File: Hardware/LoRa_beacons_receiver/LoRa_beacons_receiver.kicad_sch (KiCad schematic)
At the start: 44 parts, among them J1 Conn_Coaxial, J2 USB_C_Receptacle_USB2.0_16P, J3 I2C_Display, J4 ST-Link, J5 1PPS_out, J6 Conn_02x09_Counter_Clockwise, SW1 RST_button, SW2 BOOT_button, U1 Wio-E5, U2 CP2102N-Axx-xQFN28, U3 AP2112K-3.3, U5 74LVC1G17

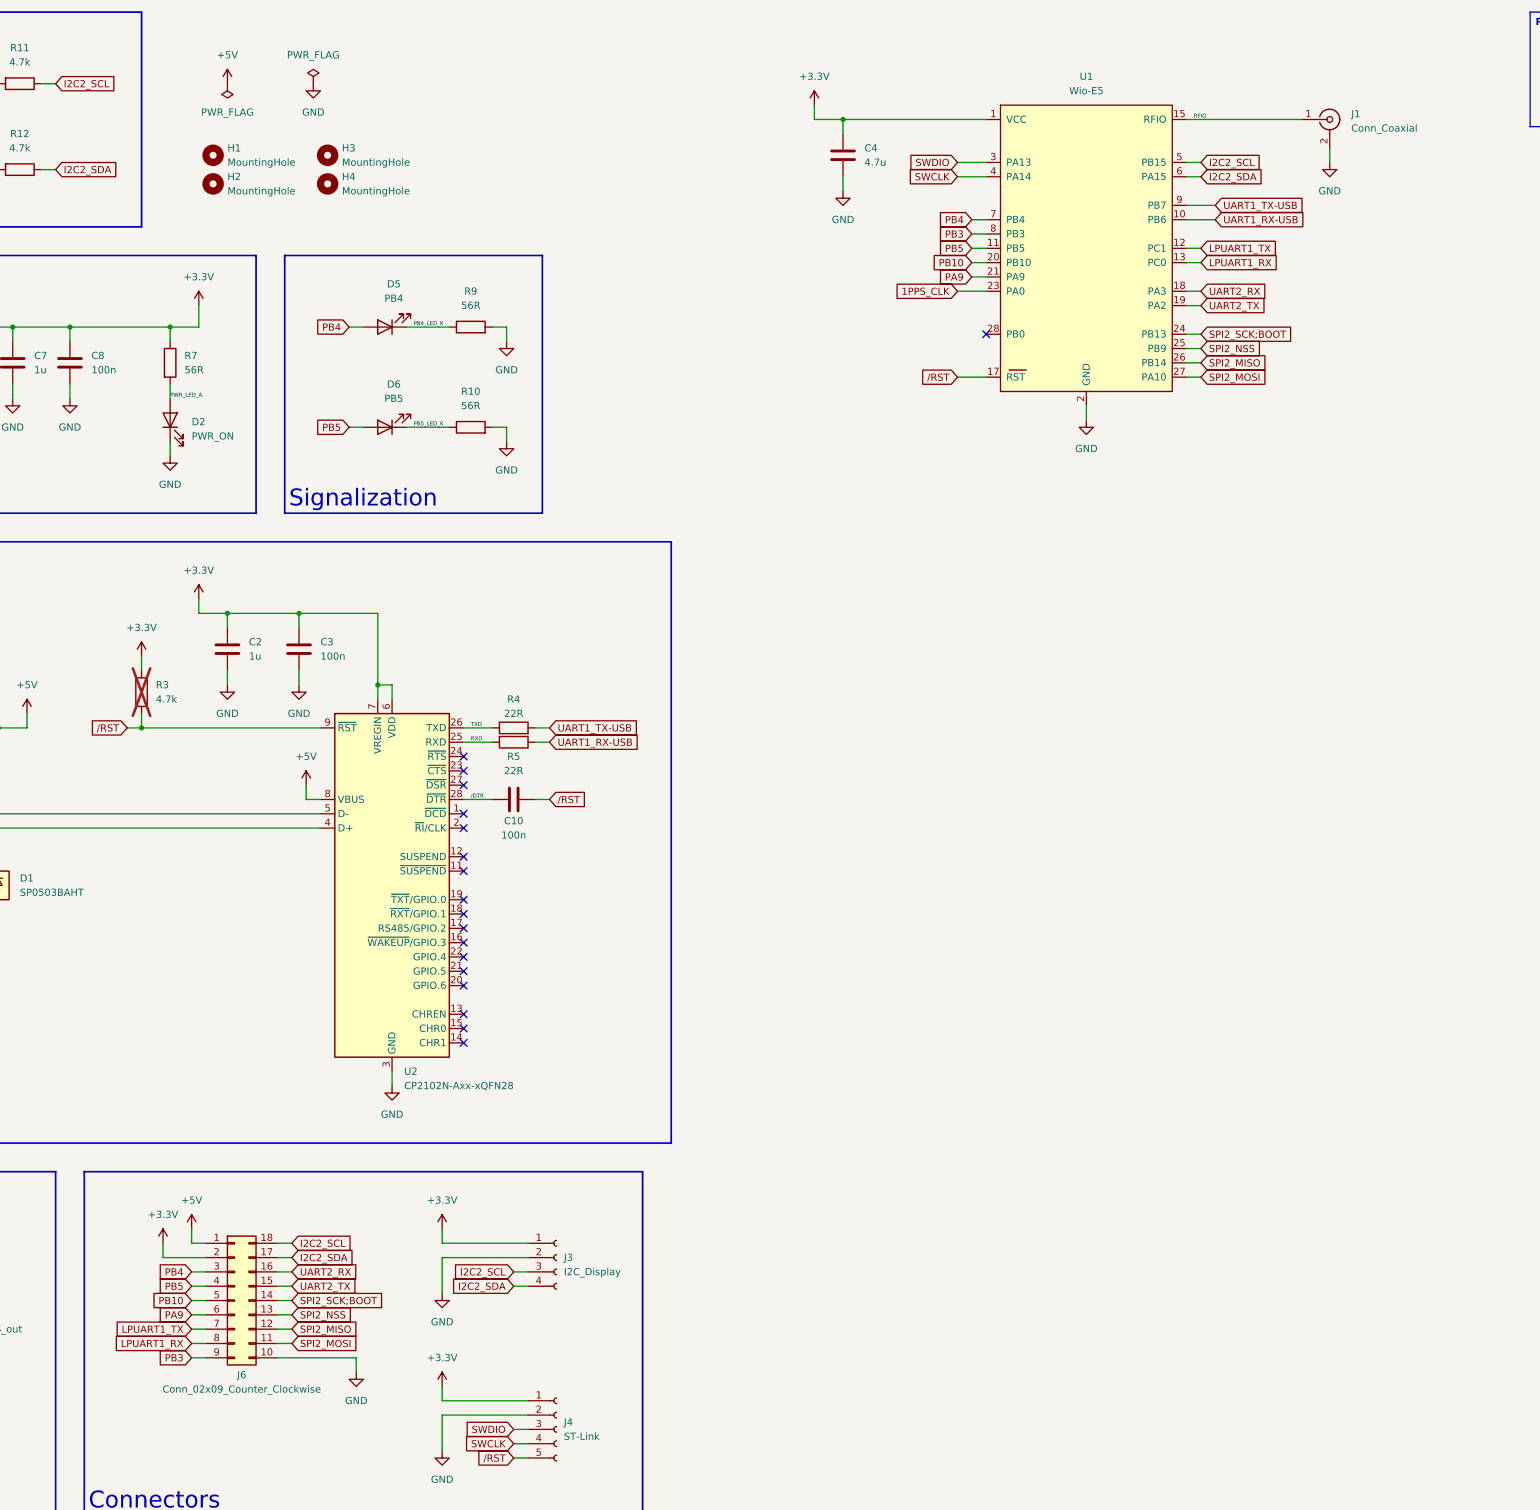
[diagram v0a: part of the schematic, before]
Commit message: First version of completely routed PCB
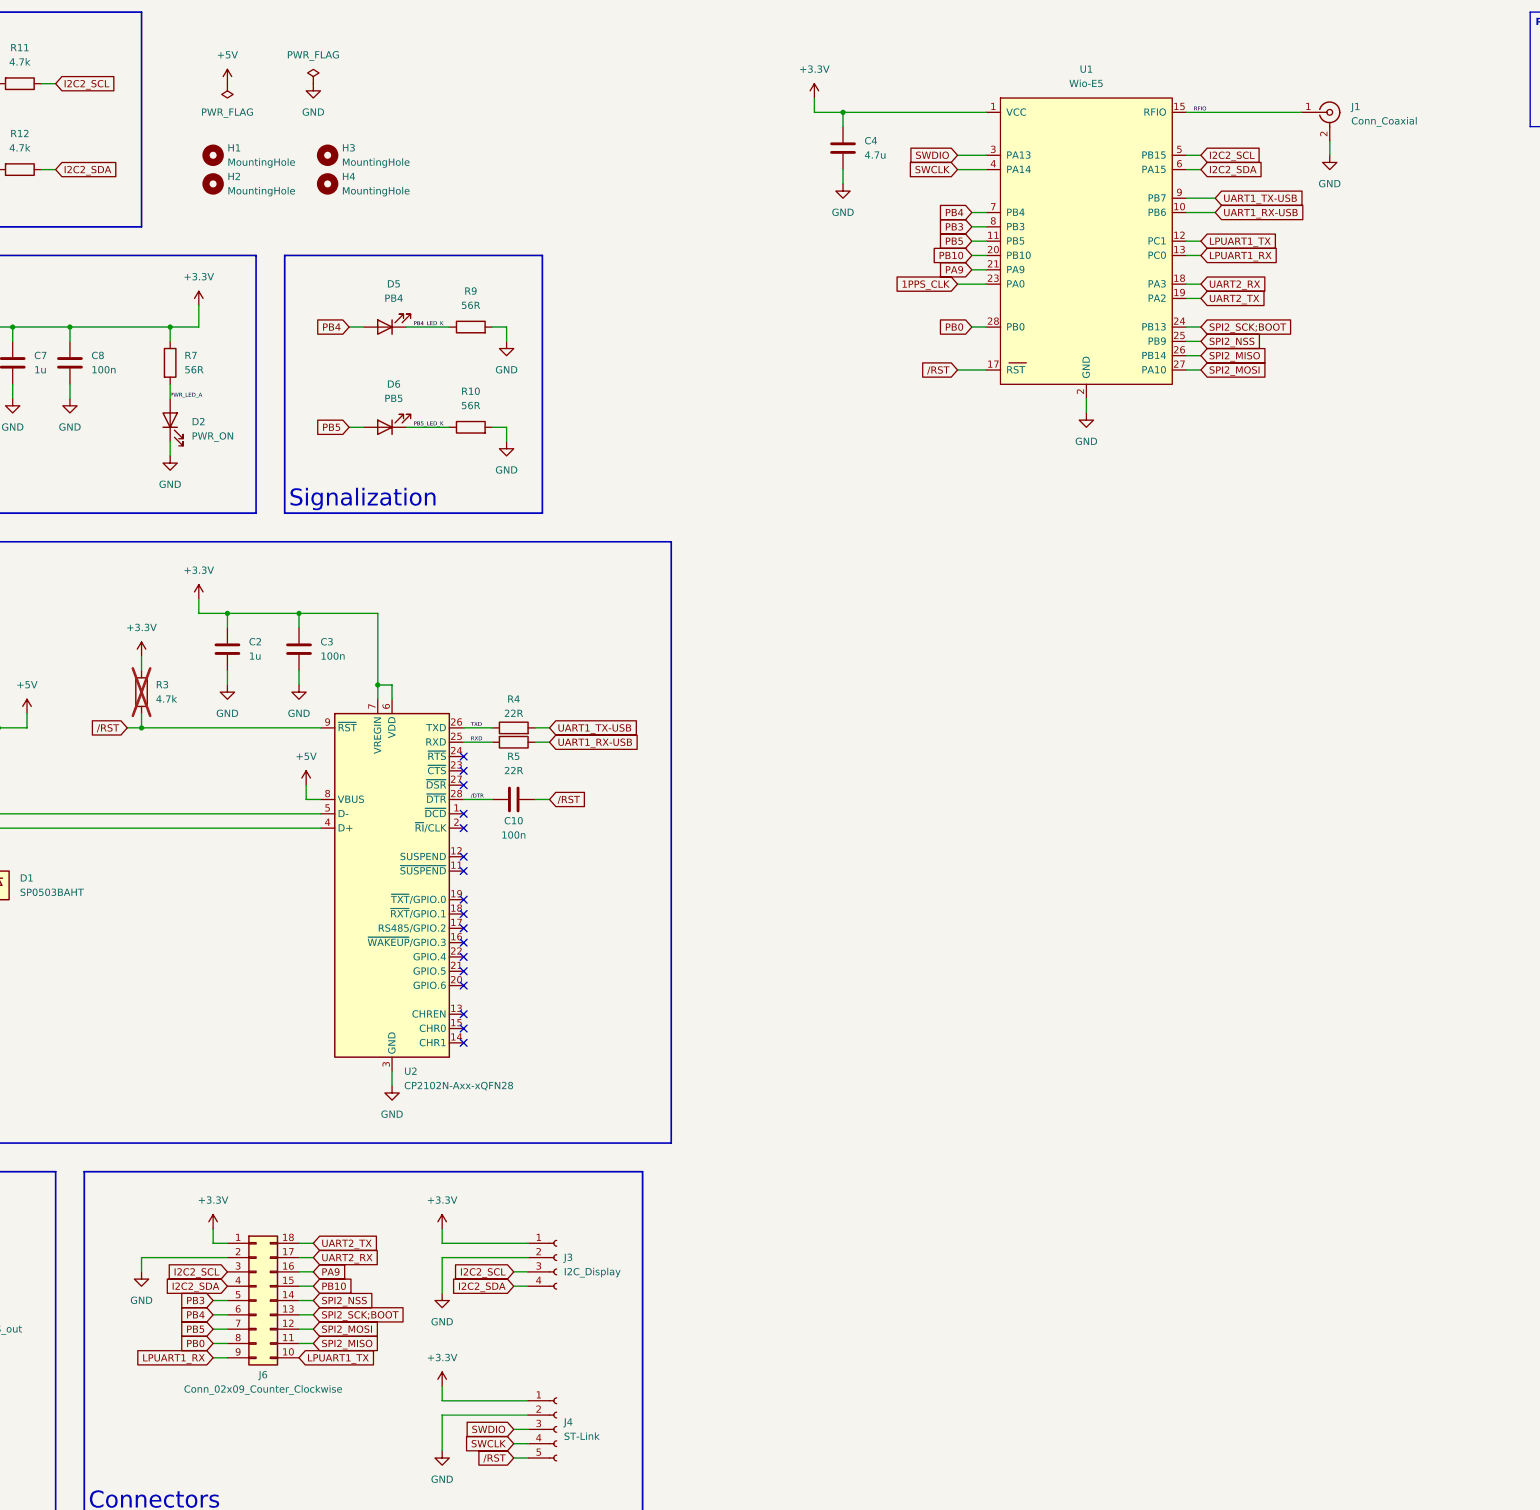
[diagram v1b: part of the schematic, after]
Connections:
- net +3.3V: now also J6.1 (Pin_1); no longer J6.2 (Pin_2)
- net +5V: no longer J6.1 (Pin_1)
- net GND: now also J6.2 (Pin_2); no longer J6.10 (Pin_10)
- net I2C2_SCL: now also J6.3 (Pin_3); no longer J6.18 (Pin_18)
- net I2C2_SDA: now also J6.4 (Pin_4); no longer J6.17 (Pin_17)
- net LPUART1_RX: now also J6.9 (Pin_9); no longer J6.8 (Pin_8)
- net LPUART1_TX: now also J6.10 (Pin_10); no longer J6.7 (Pin_7)
- net PA9: now also J6.16 (Pin_16); no longer J6.6 (Pin_6)
- net PB10: now also J6.15 (Pin_15); no longer J6.5 (Pin_5)
- net PB3: now also J6.5 (Pin_5); no longer J6.9 (Pin_9)
- net PB4: now also J6.6 (Pin_6); no longer J6.3 (Pin_3)
- net PB5: now also J6.7 (Pin_7); no longer J6.4 (Pin_4)
- net SPI2_MISO: now also J6.11 (Pin_11); no longer J6.12 (Pin_12)
- net SPI2_MOSI: now also J6.12 (Pin_12); no longer J6.11 (Pin_11)
- net SPI2_NSS: now also J6.14 (Pin_14); no longer J6.13 (Pin_13)
- net SPI2_SCK;BOOT: now also J6.13 (Pin_13); no longer J6.14 (Pin_14)
- net UART2_RX: now also J6.17 (Pin_17); no longer J6.16 (Pin_16)
- net UART2_TX: now also J6.18 (Pin_18); no longer J6.15 (Pin_15)
- net PB0: now reaches U1.28 (PB0)
- net PB0: now also J6.8 (Pin_8)
- no-connect marks 20 -> 19
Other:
- moved on the sheet: C4, J1, J6, U1

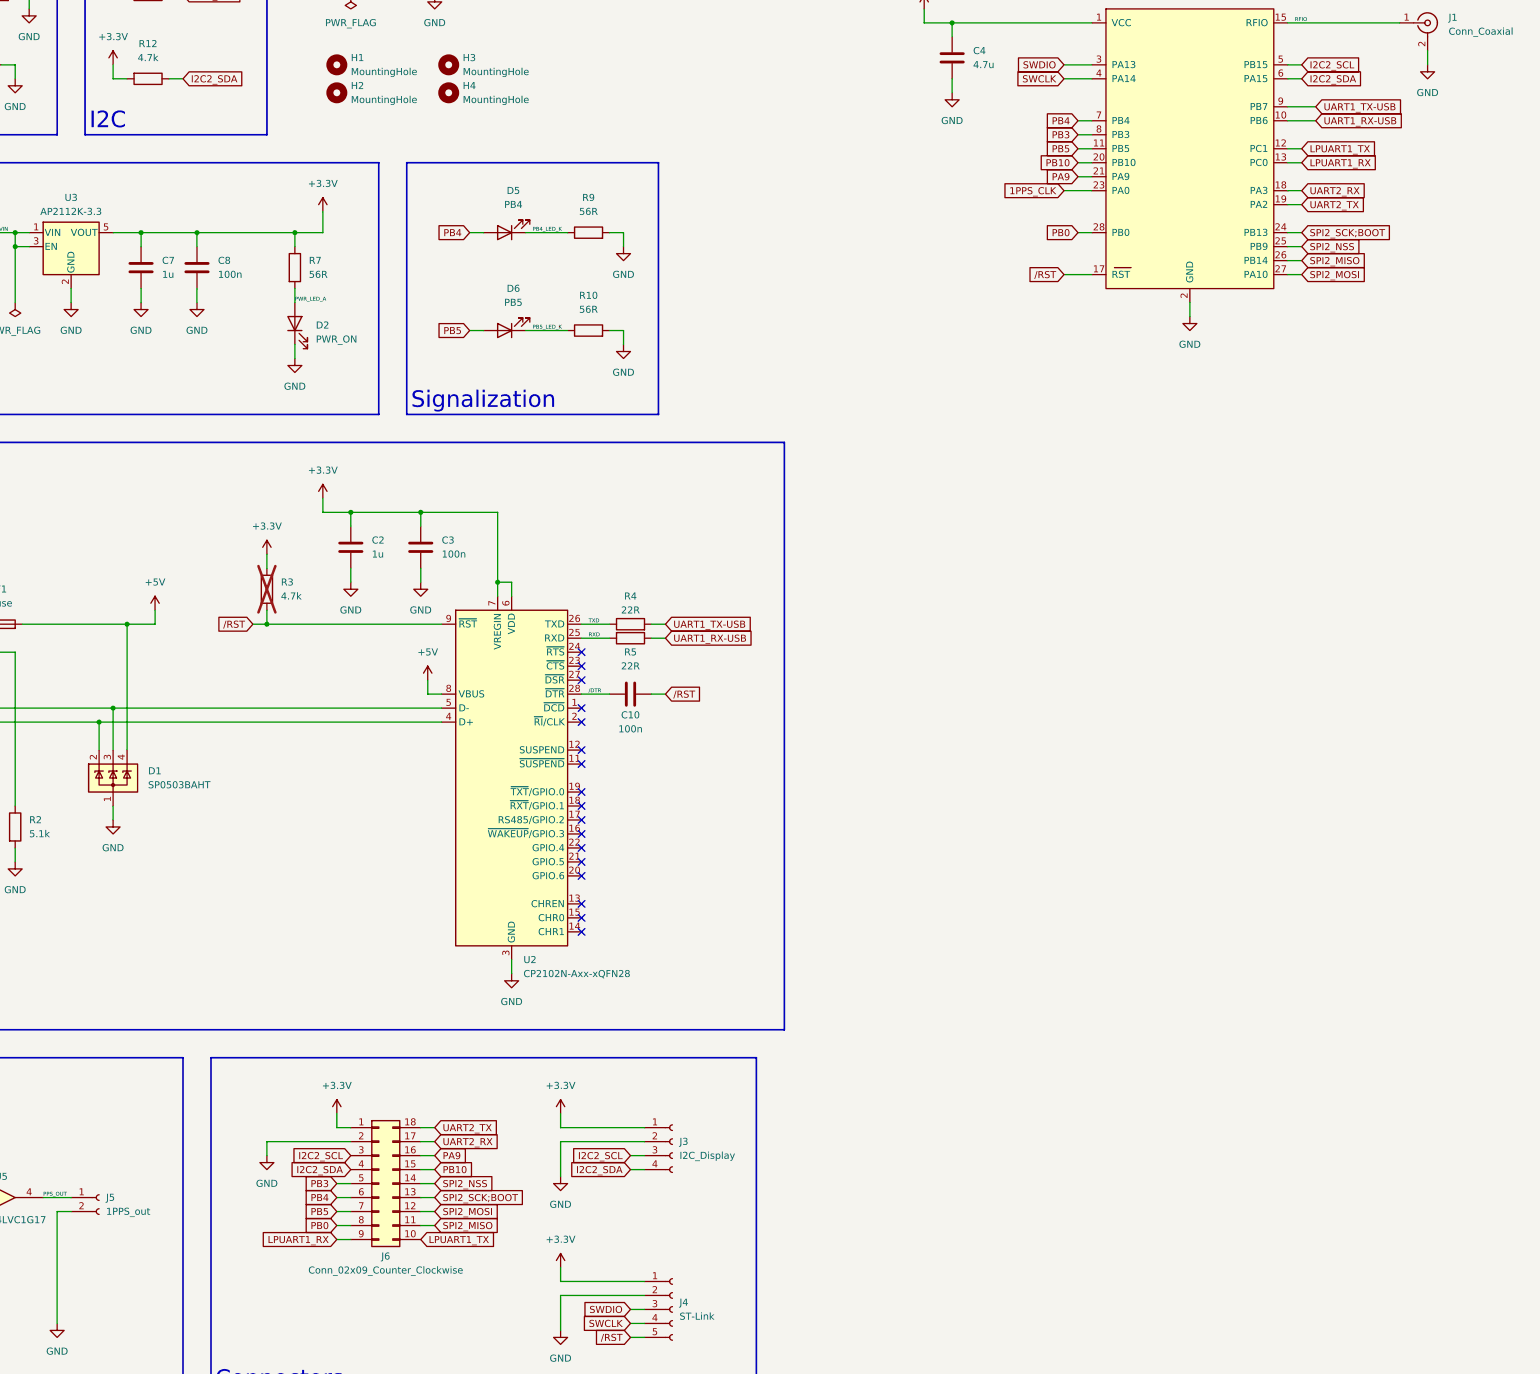
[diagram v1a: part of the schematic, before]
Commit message: Minor changes
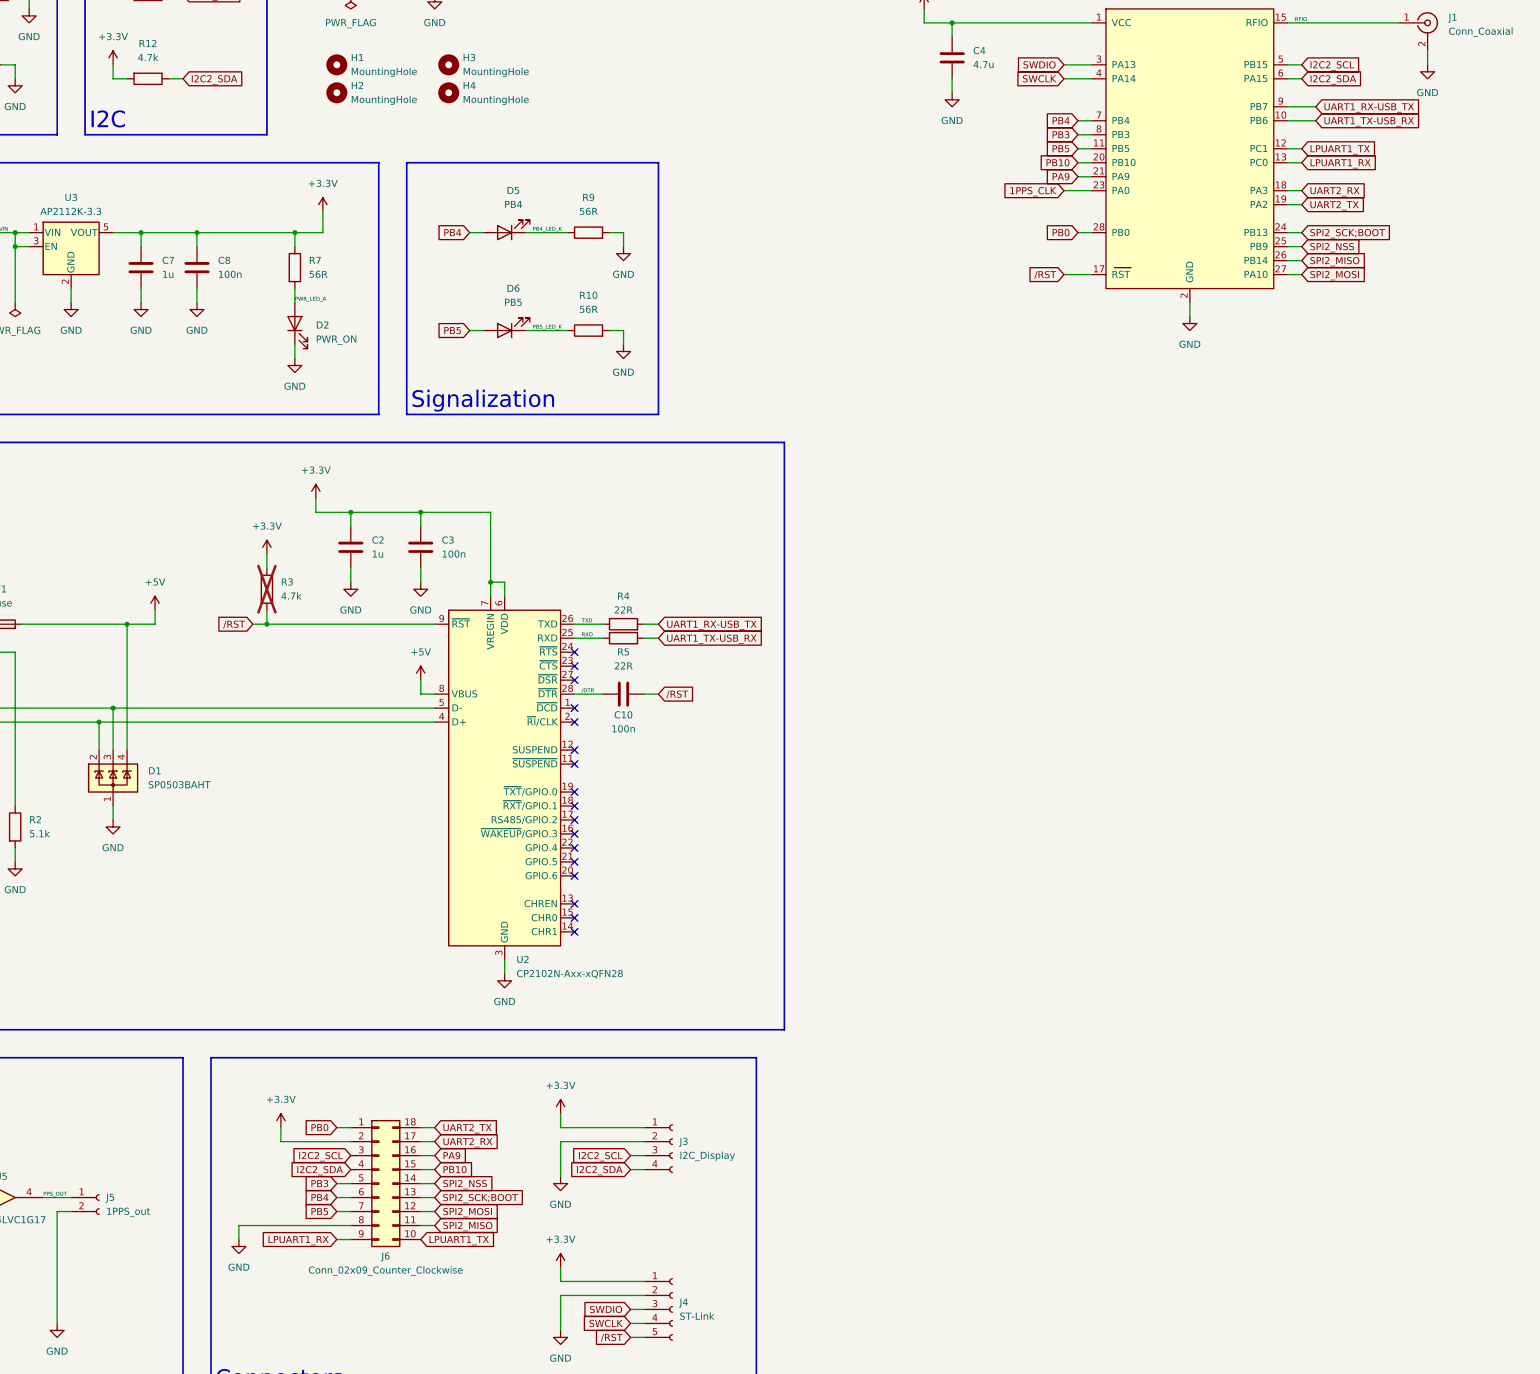
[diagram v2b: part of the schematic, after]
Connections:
- net +3.3V: now also J6.2 (Pin_2); no longer J6.1 (Pin_1)
- net GND: now also J6.8 (Pin_8); no longer J6.2 (Pin_2)
- net PB0: now also J6.1 (Pin_1); no longer J6.8 (Pin_8)
- net UART1_RX-USB renamed UART1_TX-USB_RX
- net UART1_TX-USB renamed UART1_RX-USB_TX
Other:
- moved on the sheet: C10, R4, R5, U2
